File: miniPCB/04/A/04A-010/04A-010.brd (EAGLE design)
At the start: 29 parts

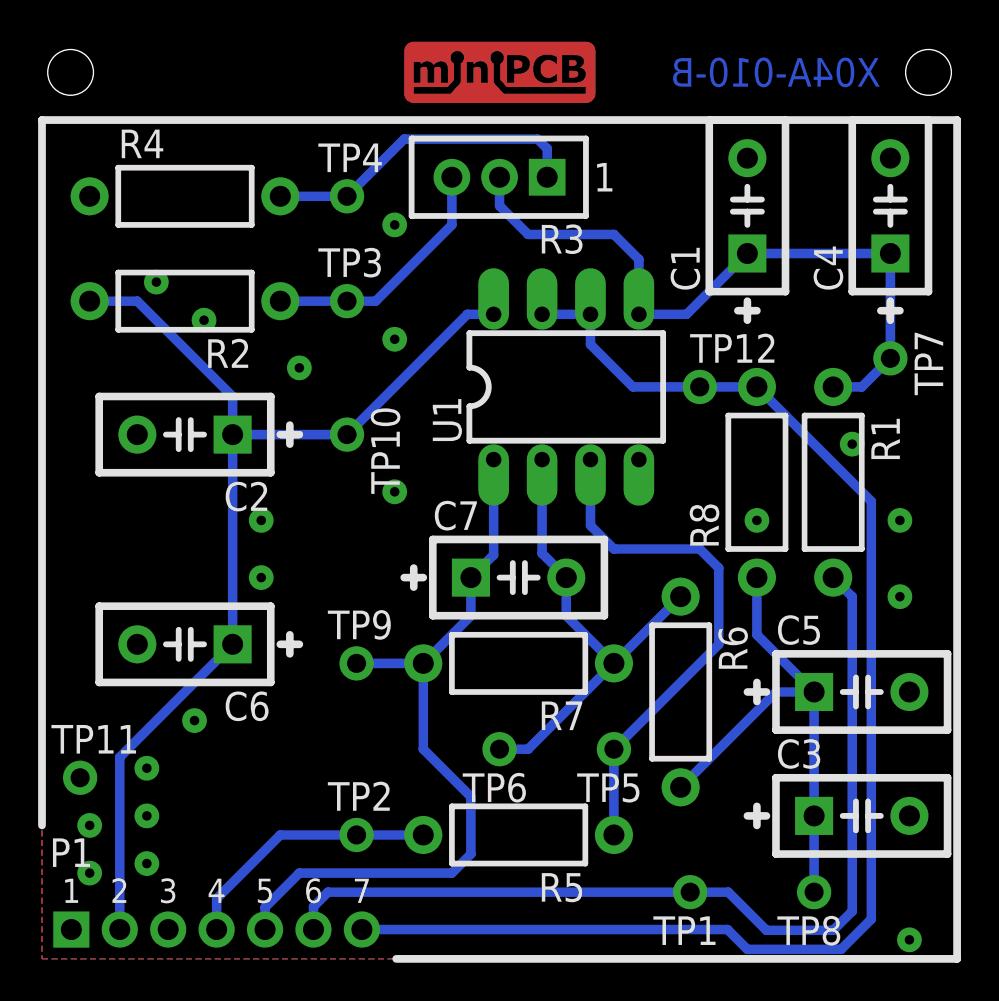
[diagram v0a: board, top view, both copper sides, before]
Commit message: NM.03SEP2023
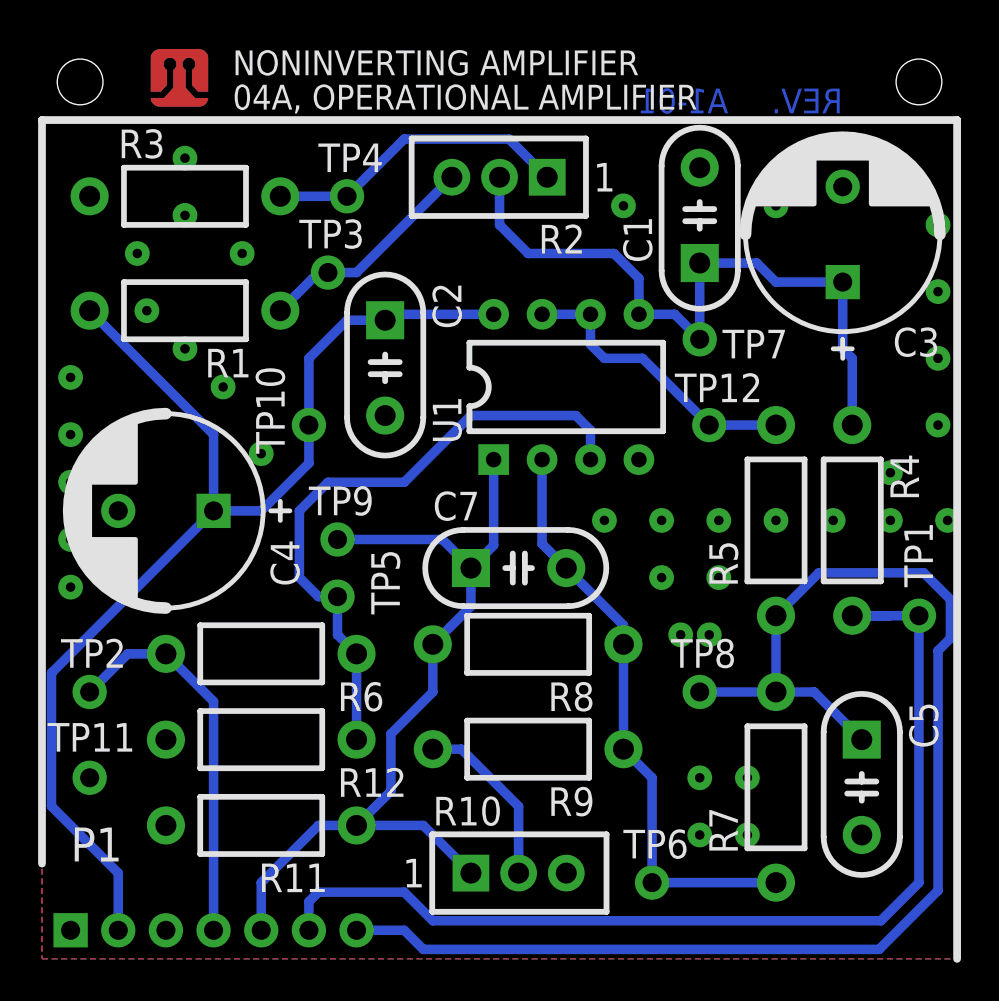
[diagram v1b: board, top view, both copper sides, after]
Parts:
- removed C6: (no value), minipcb:C050-024X044
- removed P1-: (no value), minipcb:MINIPCB_7P_50X50
- added P1: (no value), minipcb:PINS_1X7
- added R10: (no value), minipcb:TRIM_0100
- added R11, R12, R9: (no value), minipcb:0207/10
- added U$1: MINIPCB_50X50, minipcb:MINIPCB_0P_50X50MM
- C3, C4: device minipcb:C050-024X044 -> minipcb:C5MM
- R2: device minipcb:0207/10 -> minipcb:TRIM_0100
- R3: device minipcb:TRIM_0100 -> minipcb:0207/10
- moved C4 41.2 mm to (7.50, 24.5), turned to 180 degrees
- moved R4 38.9 mm to (43.5, 24.0), turned to 270 degrees
- moved R1 35.2 mm to (8.50, 35.0), turned to 180 degrees
- moved C3 30.5 mm to (43.0, 39.0), turned to 90 degrees
- moved R6 22.1 mm to (12.5, 17.0), turned to 180 degrees
- moved R5 21.3 mm to (39.5, 24.0), turned to 90 degrees
- moved R2 20.1 mm to (27.5, 42.0)
- moved R3 19.0 mm to (8.50, 41.0), turned to 0 degrees
- moved TP1 18.8 mm to (47.0, 19.0), turned to 0 degrees
- moved TP5 16.6 mm to (16.5, 20.0), turned to 270 degrees
- moved TP2 15.9 mm to (3.50, 15.0)
- moved R7 15.0 mm to (39.5, 10.0), turned to 90 degrees
- moved R8 14.7 mm to (26.5, 17.5), turned to 180 degrees
- moved TP8 12.1 mm to (35.5, 15.0), turned to 0 degrees
- moved C2 11.1 mm to (19.0, 32.0), turned to 270 degrees
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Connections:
- new net N$1: R10.2, R9.2
- net BIAS: now also C3.+, R2.2, R4.1; no longer C4.1, R1.1, R3.2
- net BIAS_CONTROL: now also P1.6, R4.2; no longer P1-.6, R1.2
- net GND: now also C3.-, C4.-, P1.1, R11.2, R12.2, R3.1; no longer C3.2, C4.2, C6.2, P1-.1, R4.1
- net IN: now also P1.4, R6.2; no longer P1-.4, R5.2
- net IN+: now also R12.1, R6.1; no longer R5.1
- net NC: now also P1.3; no longer P1-.3
- net OUT: now also P1.5, R10.1, R11.1, R8.2; no longer P1-.5, R7.2
- net POT.1: now also R2.1, R3.2; no longer R3.1, R4.2
- net POT.3: now also R1.1, R2.3; no longer R2.1, R3.3
- net V+: now also C4.+, P1.2, R1.2; no longer C6.1, P1-.2, R2.2
- net VFB: now also R8.1, R9.1; no longer R6.1
- net VREF: now also R5.2; no longer P1-.7, R8.2
- net VREF_FILTERED: now also P1.7, R5.1, R7.2; no longer C3.1, R6.2, R8.1
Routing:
- net VREF: track 72.0 -> 15.6 mm
- net VREF_FILTERED: track 26.8 -> 71.9 mm
- net N$1: track 0.00 -> 9.24 mm
- net IN: track 13.8 -> 20.4 mm
- net V+: track 56.3 -> 62.3 mm
- net VFB: track 25.1 -> 31.1 mm
- net BIAS_CONTROL: track 48.9 -> 54.7 mm
- net OUT: track 39.9 -> 45.6 mm
- net IN+: track 27.4 -> 33.0 mm
- net POT.3: track 13.2 -> 11.9 mm
- net POT.1: track 16.9 -> 16.1 mm
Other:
- board text added: "R10"
- board text added: "R11"
- board text added: "R12"
- board text added: "R9"
- board text removed: "C6"
- board text removed: "NON-INVERTING AMPLIFIER"
